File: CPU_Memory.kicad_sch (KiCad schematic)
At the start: 3 parts

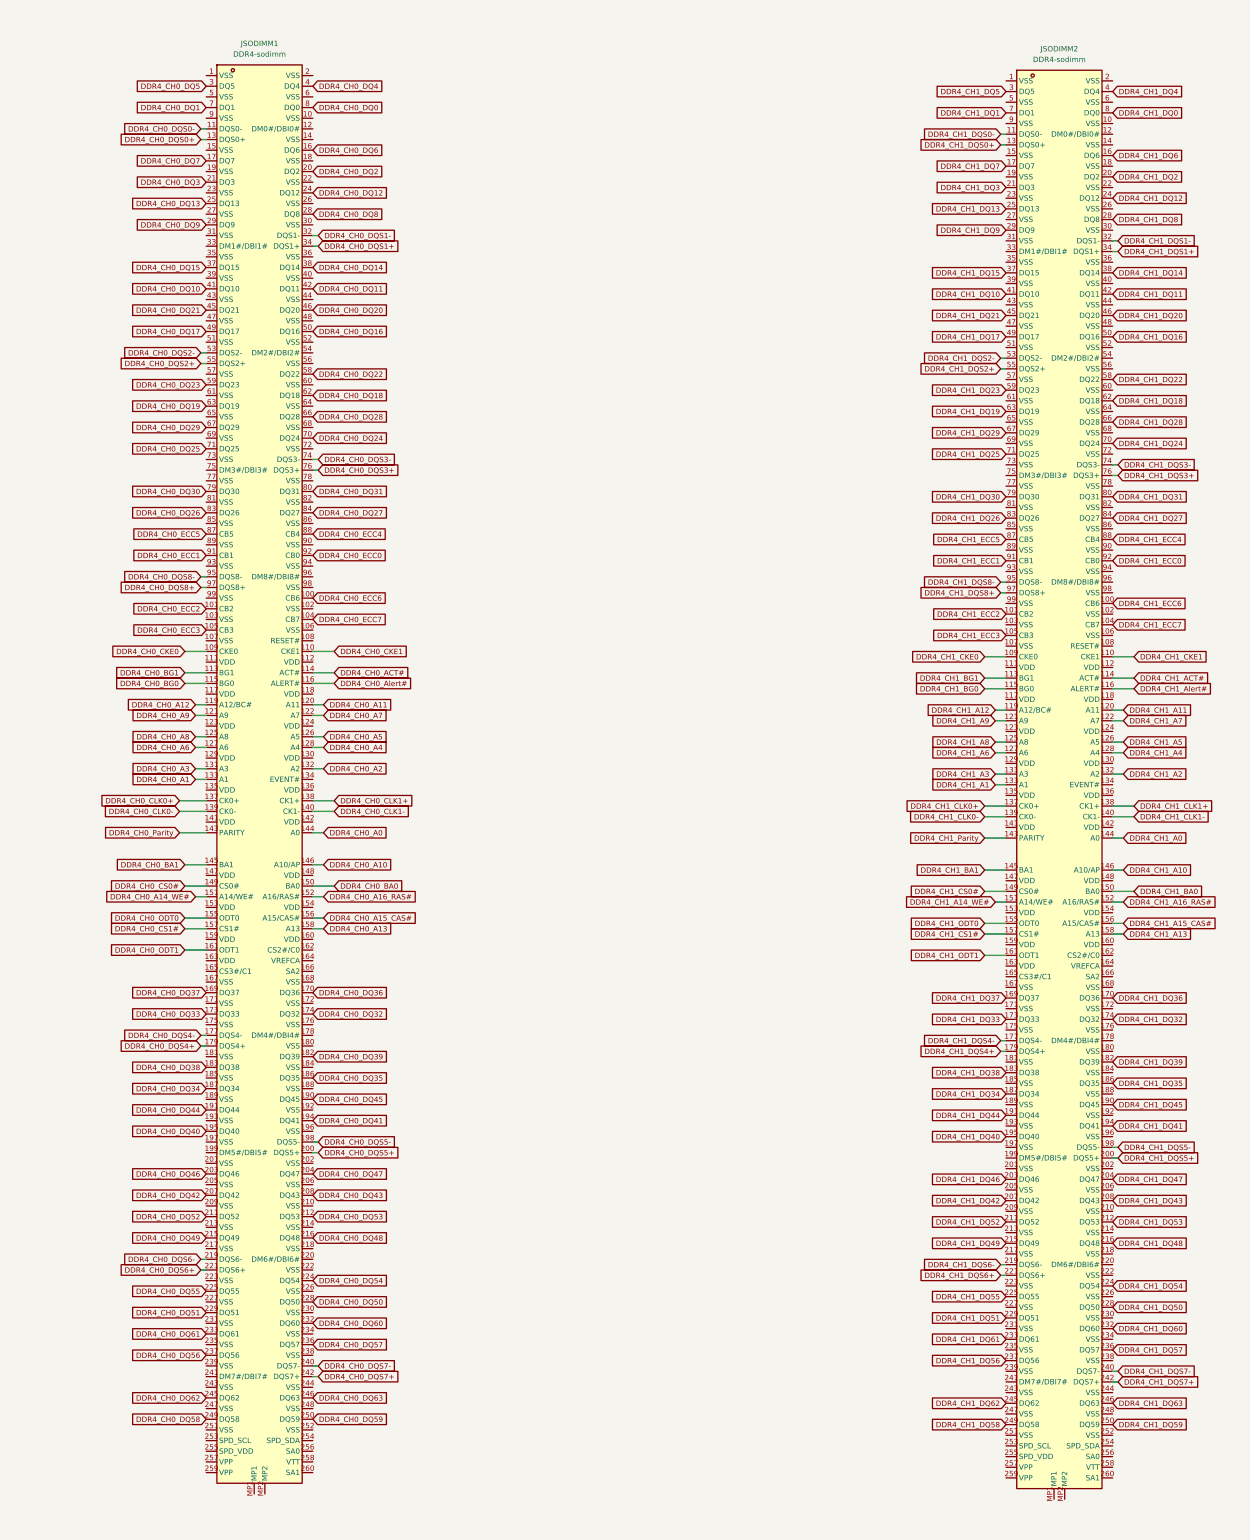
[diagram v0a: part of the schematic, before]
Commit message: Added pretty colors
pretty fun to do
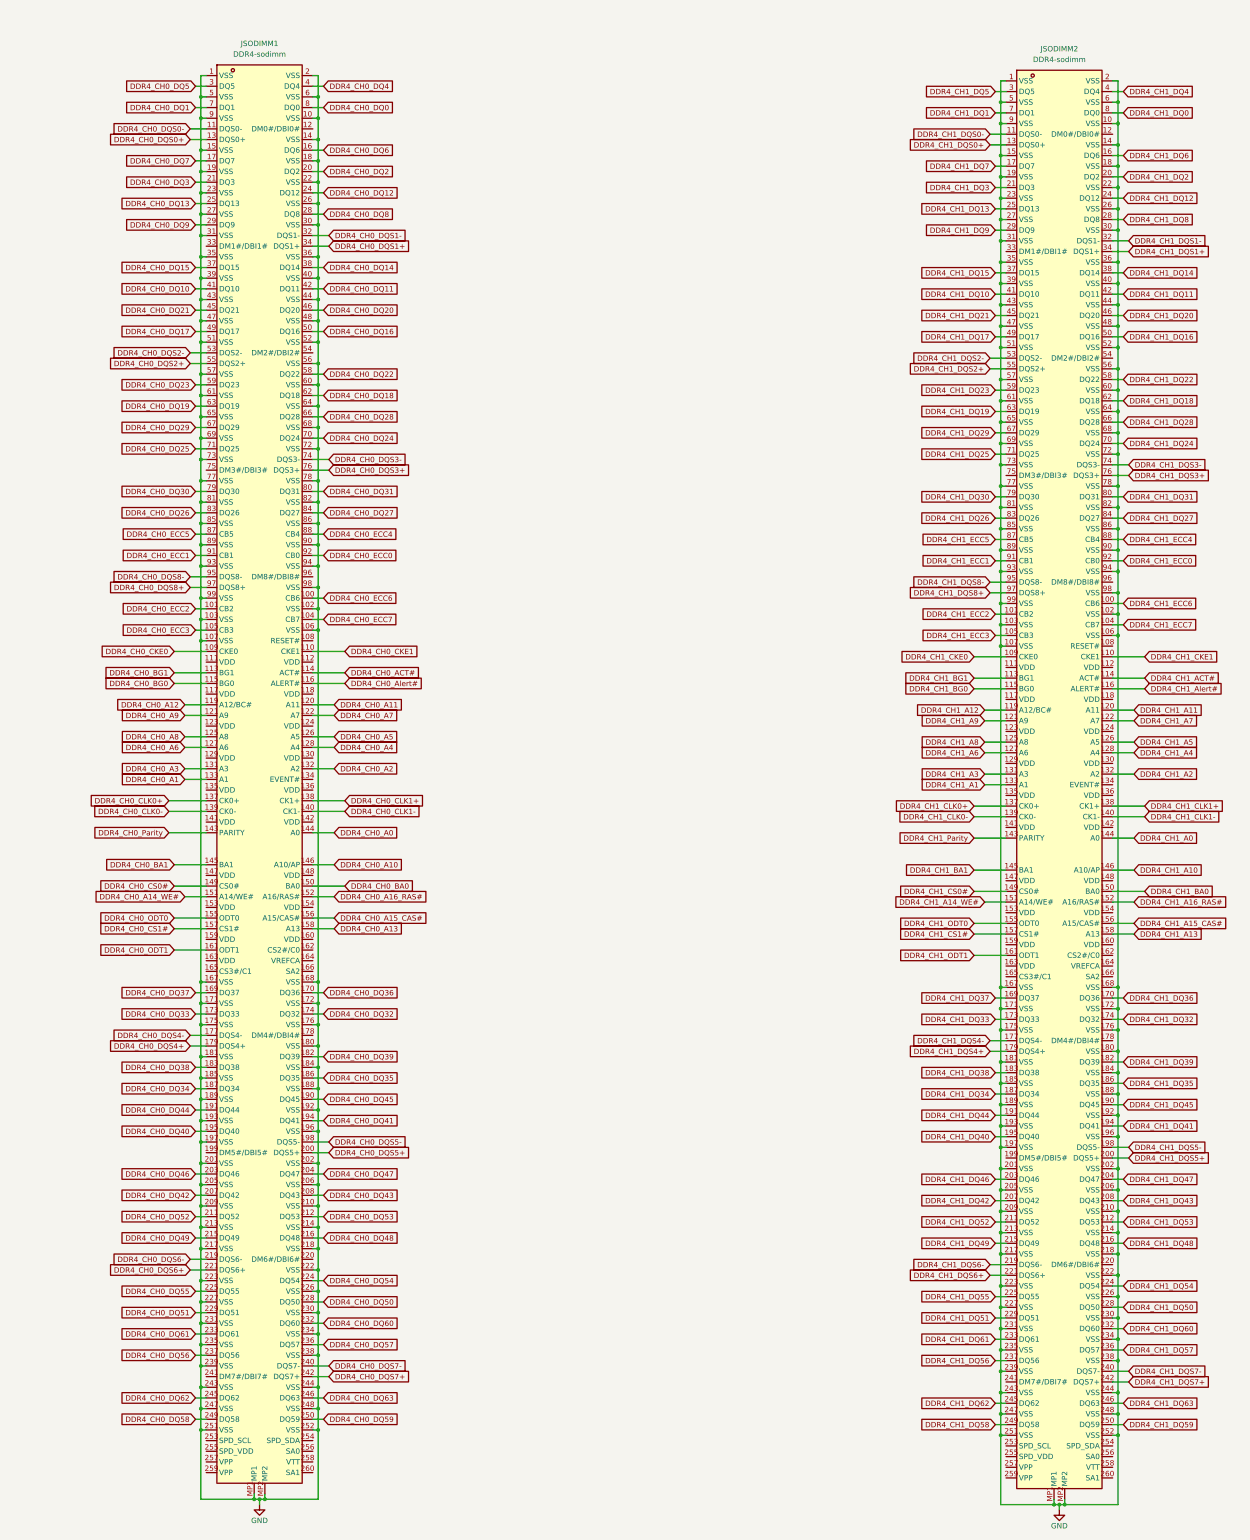
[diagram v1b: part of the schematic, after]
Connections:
- net GND: now reaches JSODIMM2.1 (VSS)
- net GND: now also JSODIMM1.1 (VSS), JSODIMM1.10 (VSS), JSODIMM1.102 (VSS), JSODIMM1.103 (VSS), JSODIMM1.106 (VSS), JSODIMM1.107 (VSS), JSODIMM1.14 (VSS), JSODIMM1.15 (VSS), JSODIMM1.167 (VSS), JSODIMM1.168 (VSS), JSODIMM1.171 (VSS), JSODIMM1.172 (VSS), JSODIMM1.175 (VSS), JSODIMM1.176 (VSS), JSODIMM1.18 (VSS), JSODIMM1.180 (VSS), JSODIMM1.181 (VSS), JSODIMM1.184 (VSS), JSODIMM1.185 (VSS), JSODIMM1.188 (VSS), JSODIMM1.189 (VSS), JSODIMM1.19 (VSS), JSODIMM1.192 (VSS), JSODIMM1.193 (VSS), JSODIMM1.196 (VSS), JSODIMM1.197 (VSS), JSODIMM1.2 (VSS), JSODIMM1.201 (VSS), JSODIMM1.202 (VSS), JSODIMM1.205 (VSS), JSODIMM1.206 (VSS), JSODIMM1.209 (VSS), JSODIMM1.210 (VSS), JSODIMM1.213 (VSS), JSODIMM1.214 (VSS), JSODIMM1.217 (VSS), JSODIMM1.218 (VSS), JSODIMM1.22 (VSS), JSODIMM1.222 (VSS), JSODIMM1.223 (VSS), JSODIMM1.226 (VSS), JSODIMM1.227 (VSS), JSODIMM1.23 (VSS), JSODIMM1.230 (VSS), JSODIMM1.231 (VSS), JSODIMM1.234 (VSS), JSODIMM1.235 (VSS), JSODIMM1.238 (VSS), JSODIMM1.239 (VSS), JSODIMM1.243 (VSS), JSODIMM1.244 (VSS), JSODIMM1.247 (VSS), JSODIMM1.248 (VSS), JSODIMM1.251 (VSS), JSODIMM1.252 (VSS), JSODIMM1.26 (VSS), JSODIMM1.27 (VSS), JSODIMM1.30 (VSS), JSODIMM1.31 (VSS), JSODIMM1.35 (VSS), JSODIMM1.36 (VSS), JSODIMM1.39 (VSS), JSODIMM1.40 (VSS), JSODIMM1.43 (VSS), JSODIMM1.44 (VSS), JSODIMM1.47 (VSS), JSODIMM1.48 (VSS), JSODIMM1.5 (VSS), JSODIMM1.51 (VSS), JSODIMM1.52 (VSS), JSODIMM1.56 (VSS), JSODIMM1.57 (VSS), JSODIMM1.6 (VSS), JSODIMM1.60 (VSS), JSODIMM1.61 (VSS), JSODIMM1.64 (VSS), JSODIMM1.65 (VSS), JSODIMM1.68 (VSS), JSODIMM1.69 (VSS), JSODIMM1.72 (VSS), JSODIMM1.73 (VSS), JSODIMM1.77 (VSS), JSODIMM1.78 (VSS), JSODIMM1.81 (VSS), JSODIMM1.82 (VSS), JSODIMM1.85 (VSS), JSODIMM1.86 (VSS), JSODIMM1.89 (VSS), JSODIMM1.9 (VSS), JSODIMM1.90 (VSS), JSODIMM1.93 (VSS), JSODIMM1.94 (VSS), JSODIMM1.98 (VSS), JSODIMM1.99 (VSS), JSODIMM1.MP1, JSODIMM1.MP2, JSODIMM2.10 (VSS), JSODIMM2.102 (VSS), JSODIMM2.103 (VSS), JSODIMM2.106 (VSS), JSODIMM2.107 (VSS), JSODIMM2.14 (VSS), JSODIMM2.15 (VSS), JSODIMM2.167 (VSS), JSODIMM2.168 (VSS), JSODIMM2.171 (VSS), JSODIMM2.172 (VSS), JSODIMM2.175 (VSS), JSODIMM2.176 (VSS), JSODIMM2.18 (VSS), JSODIMM2.180 (VSS), JSODIMM2.181 (VSS), JSODIMM2.184 (VSS), JSODIMM2.185 (VSS), JSODIMM2.188 (VSS), JSODIMM2.189 (VSS), JSODIMM2.19 (VSS), JSODIMM2.192 (VSS), JSODIMM2.193 (VSS), JSODIMM2.196 (VSS), JSODIMM2.197 (VSS), JSODIMM2.2 (VSS), JSODIMM2.201 (VSS), JSODIMM2.202 (VSS), JSODIMM2.205 (VSS), JSODIMM2.206 (VSS), JSODIMM2.209 (VSS), JSODIMM2.210 (VSS), JSODIMM2.213 (VSS), JSODIMM2.214 (VSS), JSODIMM2.217 (VSS), JSODIMM2.218 (VSS), JSODIMM2.22 (VSS), JSODIMM2.222 (VSS), JSODIMM2.223 (VSS), JSODIMM2.226 (VSS), JSODIMM2.227 (VSS), JSODIMM2.23 (VSS), JSODIMM2.230 (VSS), JSODIMM2.231 (VSS), JSODIMM2.234 (VSS), JSODIMM2.235 (VSS), JSODIMM2.238 (VSS), JSODIMM2.239 (VSS), JSODIMM2.243 (VSS), JSODIMM2.244 (VSS), JSODIMM2.247 (VSS), JSODIMM2.248 (VSS), JSODIMM2.251 (VSS), JSODIMM2.252 (VSS), JSODIMM2.26 (VSS), JSODIMM2.27 (VSS), JSODIMM2.30 (VSS), JSODIMM2.31 (VSS), JSODIMM2.35 (VSS), JSODIMM2.36 (VSS), JSODIMM2.39 (VSS), JSODIMM2.40 (VSS), JSODIMM2.43 (VSS), JSODIMM2.44 (VSS), JSODIMM2.47 (VSS), JSODIMM2.48 (VSS), JSODIMM2.5 (VSS), JSODIMM2.51 (VSS), JSODIMM2.52 (VSS), JSODIMM2.56 (VSS), JSODIMM2.57 (VSS), JSODIMM2.6 (VSS), JSODIMM2.60 (VSS), JSODIMM2.61 (VSS), JSODIMM2.64 (VSS), JSODIMM2.65 (VSS), JSODIMM2.68 (VSS), JSODIMM2.69 (VSS), JSODIMM2.72 (VSS), JSODIMM2.73 (VSS), JSODIMM2.77 (VSS), JSODIMM2.78 (VSS), JSODIMM2.81 (VSS), JSODIMM2.82 (VSS), JSODIMM2.85 (VSS), JSODIMM2.86 (VSS), JSODIMM2.89 (VSS), JSODIMM2.9 (VSS), JSODIMM2.90 (VSS), JSODIMM2.93 (VSS), JSODIMM2.94 (VSS), JSODIMM2.98 (VSS), JSODIMM2.99 (VSS), JSODIMM2.MP1, JSODIMM2.MP2
